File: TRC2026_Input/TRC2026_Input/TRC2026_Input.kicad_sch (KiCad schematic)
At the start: 24 parts, among them J1 Conn_01x06_Pin, J15 Conn_01x04_Pin, J2 Conn_01x06_Pin, J22 LoRa, J23 Conn_01x12_Pin, SW1 SW_Push, SW2 SW_Push, SW3 SW_Push, SW4 SW_Push, SW5 SW_SPDT

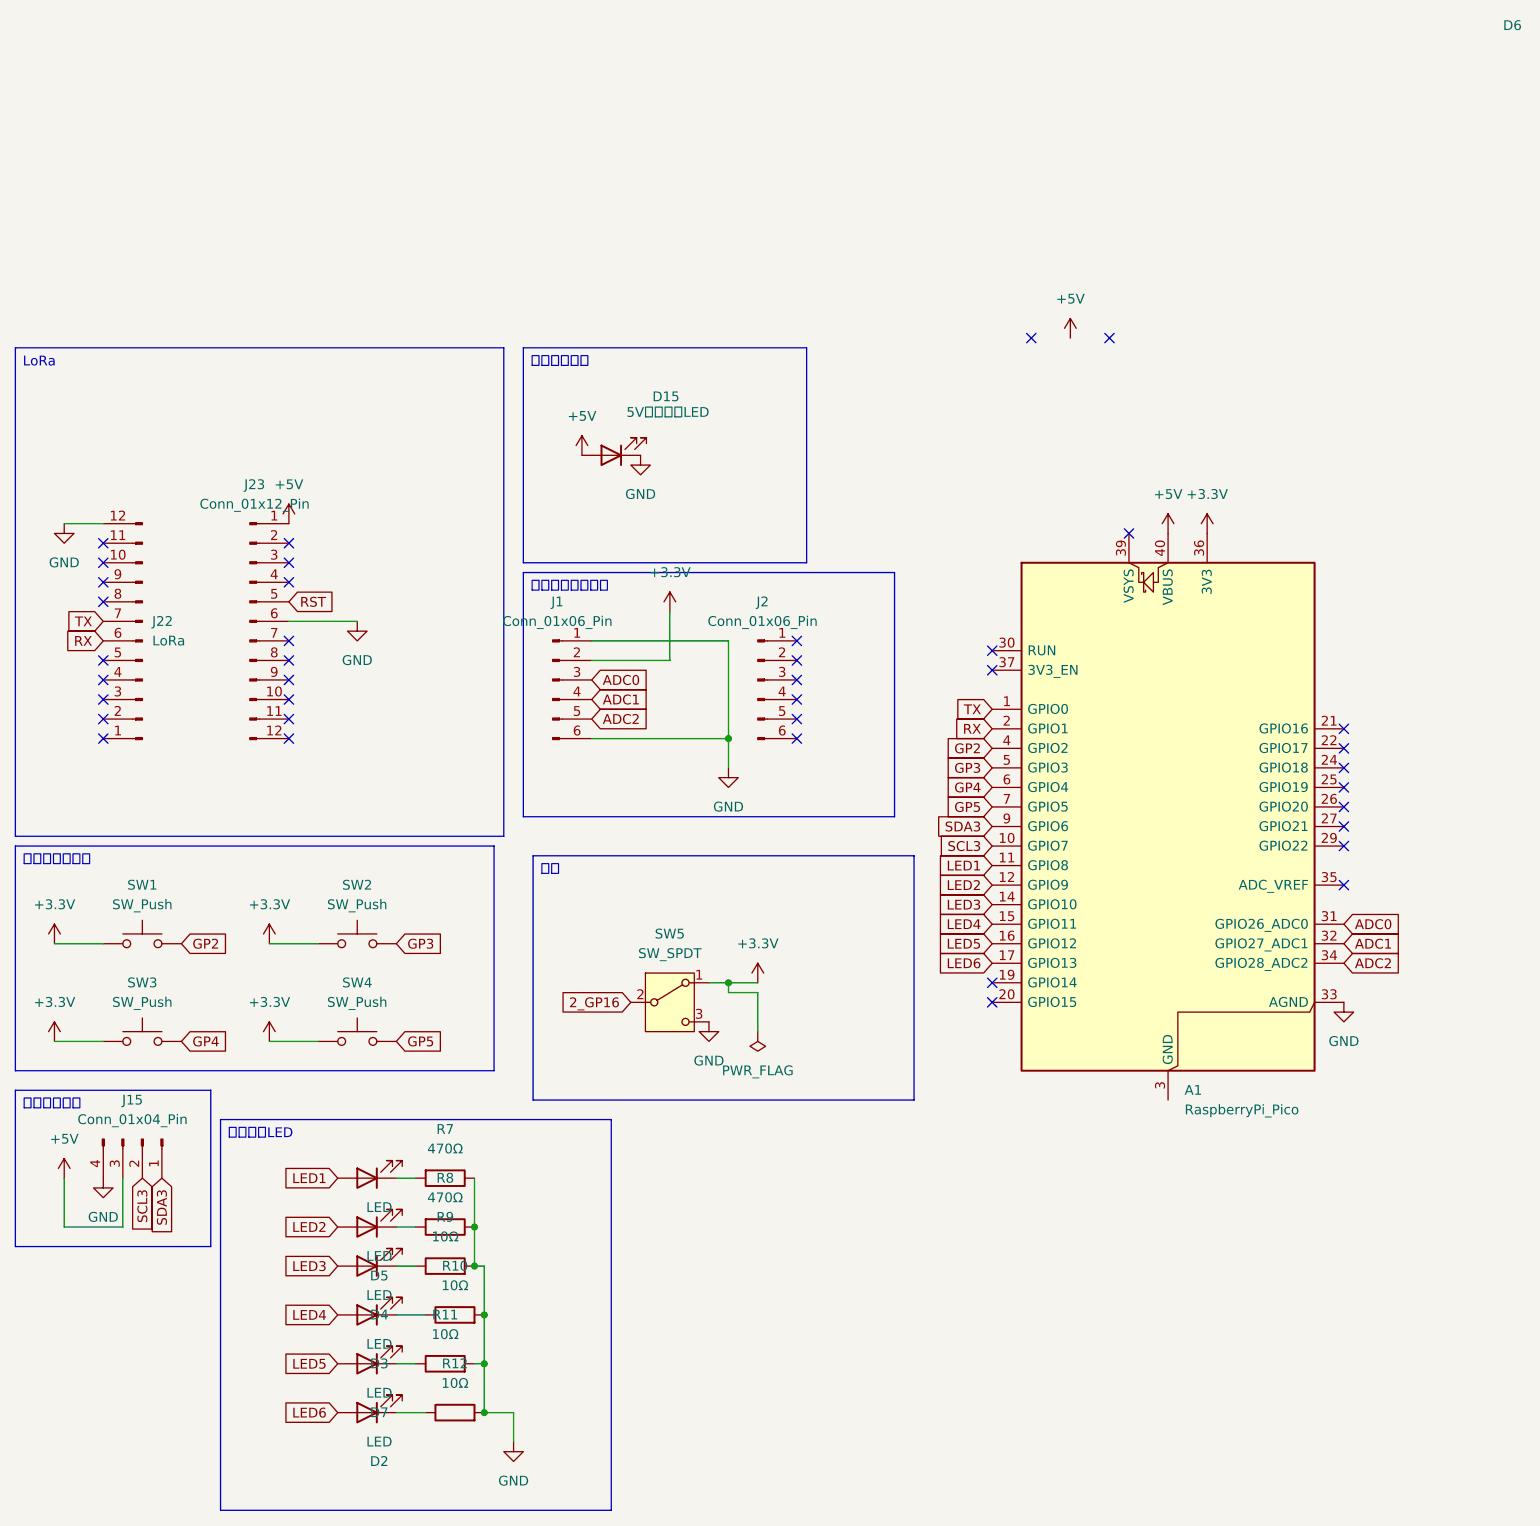
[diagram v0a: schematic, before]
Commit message: いろいろと変更
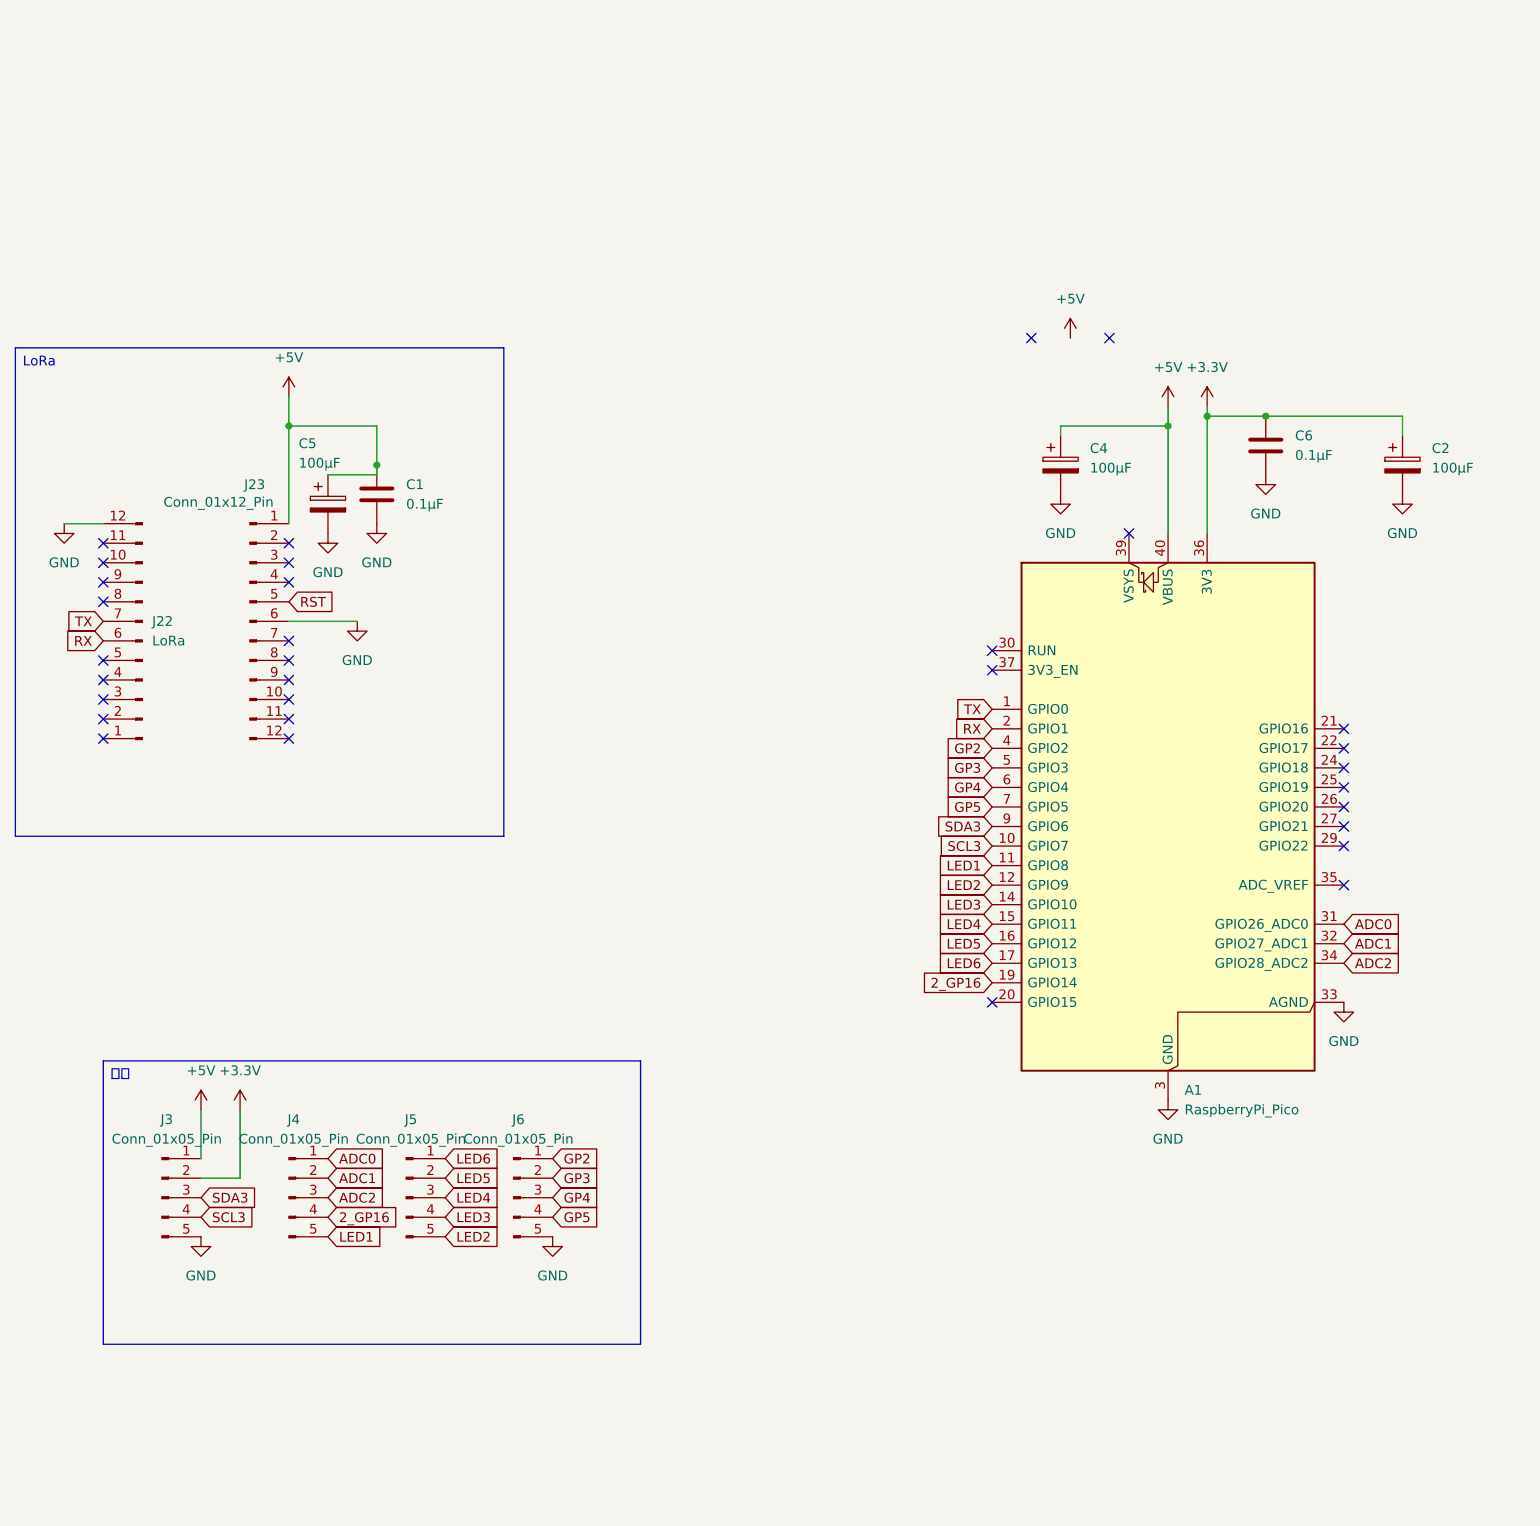
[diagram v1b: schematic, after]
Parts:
- removed D15: 5V抵抗内蔵LED, LED_THT:LED_D5.0mm, symbol Device:LED
- removed D2, D3, D4, D5, D6, D7: LED, LED_THT:LED_D5.0mm, symbol Device:LED
- removed J1, J2: Conn_01x06_Pin, symbol Connector:Conn_01x06_Pin
- removed J15: Conn_01x04_Pin, Connector_PinSocket_2.54mm:PinSocket_1x04_P2.54mm_Vertical, symbol Connector:Conn_01x04_Pin
- removed R10, R11, R12, R9: 10Ω, Resistor_THT:R_Axial_DIN0207_L6.3mm_D2.5mm_P10.16mm_Horizontal, symbol Device:R
- removed R7, R8: 470Ω, Resistor_THT:R_Axial_DIN0207_L6.3mm_D2.5mm_P10.16mm_Horizontal, symbol Device:R
- removed SW1, SW2, SW3, SW4: SW_Push, symbol Switch:SW_Push
- removed SW5: SW_SPDT, kicad_3MS1J102M2QES:3MS1J102M2QES, symbol Switch:SW_SPDT
- added C1, C6: 0.1μF, Capacitor_SMD:C_0603_1608Metric, symbol Device:C
- added C2, C4, C5: 100μF, Capacitor_THT:CP_Radial_D8.0mm_P3.50mm, symbol Device:C_Polarized
- added J3, J4, J5, J6: Conn_01x05_Pin, Connector_PinHeader_2.54mm:PinHeader_1x05_P2.54mm_Vertical, symbol Connector:Conn_01x05_Pin
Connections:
- net +3.3V: now also C2.1, C6.1, J3.2 (Pin_2)
- net +5V: now also C1.1, C4.1, C5.1, J3.1 (Pin_1)
- net 2_GP16: now also A1.19 (GPIO14), J4.4 (Pin_4)
- net ADC0: now also J4.1 (Pin_1)
- net ADC1: now also J4.2 (Pin_2)
- net ADC2: now also J4.3 (Pin_3)
- net GND: now also A1.13 (GND), A1.18 (GND), A1.23 (GND), A1.28 (GND), A1.3 (GND), A1.38 (GND), A1.8 (GND), C1.2, C2.2, C4.2, C5.2, C6.2, J3.5 (Pin_5), J6.5 (Pin_5)
- net GP2: now also J6.1 (Pin_1)
- net GP3: now also J6.2 (Pin_2)
- net GP4: now also J6.3 (Pin_3)
- net GP5: now also J6.4 (Pin_4)
- net LED1: now also J4.5 (Pin_5)
- net LED2: now also J5.5 (Pin_5)
- net LED3: now also J5.4 (Pin_4)
- net LED4: now also J5.3 (Pin_3)
- net LED5: now also J5.2 (Pin_2)
- net LED6: now also J5.1 (Pin_1)
- net SCL3: now also J3.4 (Pin_4)
- net SDA3: now also J3.3 (Pin_3)
- no-connect marks 39 -> 32
